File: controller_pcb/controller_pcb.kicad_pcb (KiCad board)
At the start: 2 copper layers, 24 x 22.1 mm, 19 parts, among them J11 IO connector, J12 LED_Pins, SW11 PEC11L-4220F-S0015, U11 ATtiny1606-M

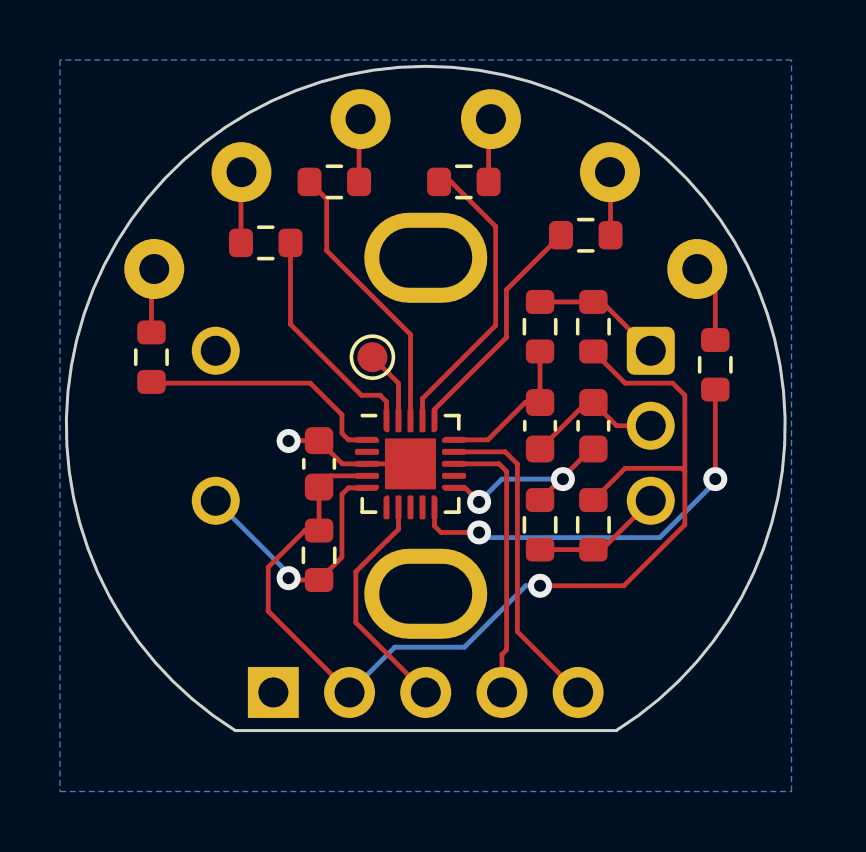
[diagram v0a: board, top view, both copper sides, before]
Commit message: v1 for manufacturing
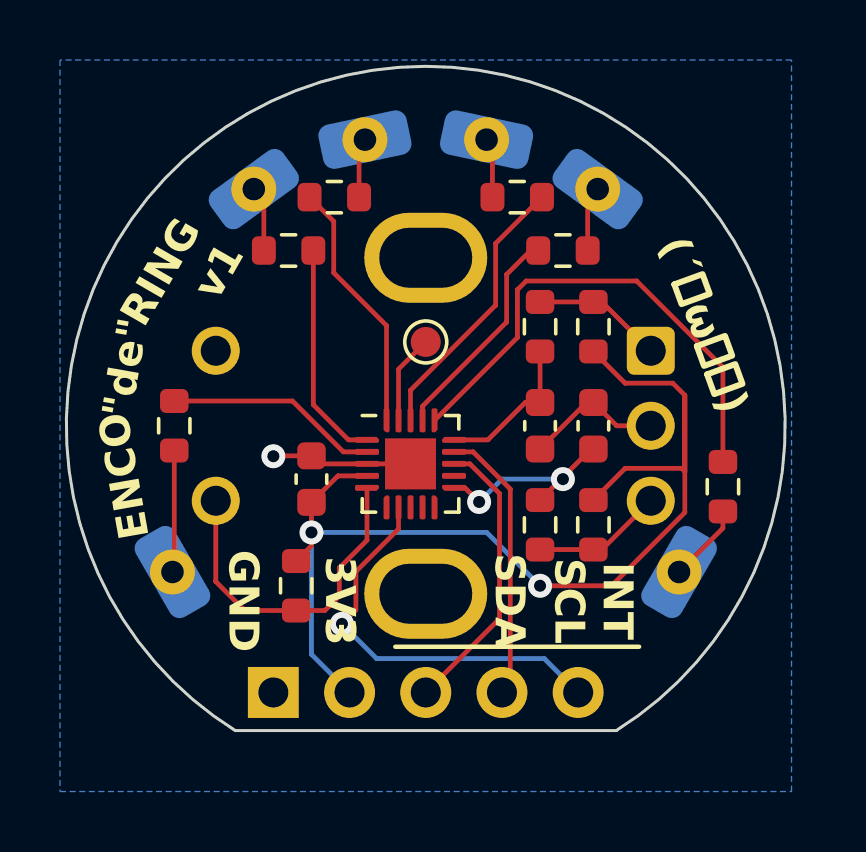
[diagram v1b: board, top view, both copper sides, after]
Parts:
- J3: renamed from J12; moved to B.Cu
- R10: renamed from R18; value 220 -> 20ohm
- R11: renamed from R17; value 220 -> 20ohm
- R12: renamed from R16; value 220 -> 20ohm
- R7: renamed from R21; value 220 -> 20ohm
- R8: renamed from R20; value 220 -> 20ohm
- R9: renamed from R19; value 220 -> 20ohm
- moved R12 4.07 mm to (60.7, 52.8), turned to -90 degrees
- moved R7 2.41 mm to (42.4, 50.8), turned to -90 degrees
- moved R10 1.85 mm to (53.8, 43.2), turned to 180 degrees
- moved TP2 1.85 mm to (50.8, 48.0)
- moved R2 1.27 mm to (46.5, 56.1)
- moved R11 0.92 mm to (55.4, 45.0)
- moved R8 0.80 mm to (46.2, 45.0)
- moved C2 0.57 mm to (47.0, 52.6)
- moved R9 0.51 mm to (47.8, 43.2)
- turned J3 to 180 degrees
- renumbered C11 to C2, C13 to C3, C12 to C4, J11 to J2, R11 to R2, R13 to R3, R12 to R4, R15 to R5, R14 to R6, SW11 to SW2, TP11 to TP2, U11 to U2
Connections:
- J2 pad 3: INT -> SDA
- J2 pad 4: SDA -> SCL
- J2 pad 5: SCL -> INT
- J3 pad 1: Net-(J12-Pin_1) -> Net-(J3-Pin_1)
- J3 pad 2: Net-(J12-Pin_2) -> Net-(J3-Pin_2)
- J3 pad 3: Net-(J12-Pin_3) -> Net-(J3-Pin_3)
- J3 pad 4: Net-(J12-Pin_4) -> Net-(J3-Pin_4)
- J3 pad 5: Net-(J12-Pin_5) -> Net-(J3-Pin_5)
- J3 pad 6: Net-(J12-Pin_6) -> Net-(J3-Pin_6)
- R10 pad 1: LED3 -> LED4
- R10 pad 2: Net-(J12-Pin_3) -> Net-(J3-Pin_4)
- R11 pad 1: LED2 -> LED5
- R11 pad 2: Net-(J12-Pin_2) -> Net-(J3-Pin_5)
- R12 pad 1: LED1 -> LED6
- R12 pad 2: Net-(J12-Pin_1) -> Net-(J3-Pin_6)
- R7 pad 1: LED6 -> LED1
- R7 pad 2: Net-(J12-Pin_6) -> Net-(J3-Pin_1)
- R8 pad 1: LED5 -> LED2
- R8 pad 2: Net-(J12-Pin_5) -> Net-(J3-Pin_2)
- R9 pad 1: LED4 -> LED3
- R9 pad 2: Net-(J12-Pin_4) -> Net-(J3-Pin_3)
- U2 pad 1: LED6 -> LED2
- U2 pad 10: LED1 -> unconnected-(U2-PB4-Pad10)
- U2 pad 16: LED2 -> LED6
- U2 pad 17: LED3 -> LED5
- U2 pad 2: unconnected-(U11-PA3-Pad2) -> LED1
- U2 pad 20: LED5 -> LED3
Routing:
- net LED6: track 8.35 -> 16.8 mm
- net LED1: track 13.9 -> 7.13 mm, vias 2 -> 0
- net INT: track 7.73 -> 13.5 mm, vias 0 -> 1
- net Net-(J3-Pin_1): track 0.00 -> 4.08 mm
- net ENCS: track 8.73 -> 11.4 mm, vias 1 -> 0
- net Net-(J3-Pin_6): track 0.00 -> 2.62 mm
- net Net-(J12-Pin_1): track 2.62 -> 0.00 mm
- net VCC: track 35.9 -> 38.3 mm, vias 1 -> 2
- net Net-(J12-Pin_5): track 2.37 -> 0.00 mm
- net Net-(J3-Pin_5): track 0.00 -> 2.18 mm
- net Net-(J3-Pin_2): track 0.00 -> 2.18 mm
- net Net-(J12-Pin_6): track 2.15 -> 0.00 mm
- net Net-(J12-Pin_3): track 2.13 -> 0.00 mm
- net Net-(J12-Pin_4): track 2.11 -> 0.00 mm
- net Net-(J12-Pin_2): track 2.11 -> 0.00 mm
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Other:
- board text added: "(´・ω・｀)"
- board text added: "3V3 GND"
- board text added: "ENCO"
- board text added: "INT SCL"
- board text added: "RING"
- board text added: "SDA"
- board text added: "pollo"
- board text added: "v1"
- board text added: "{dblquote}de{dblquote}"
